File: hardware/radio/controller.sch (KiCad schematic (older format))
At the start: 11 parts, among them IC301 ATMEGA328-P, Q301 Q_NMOS_DGS, X301 8MHz

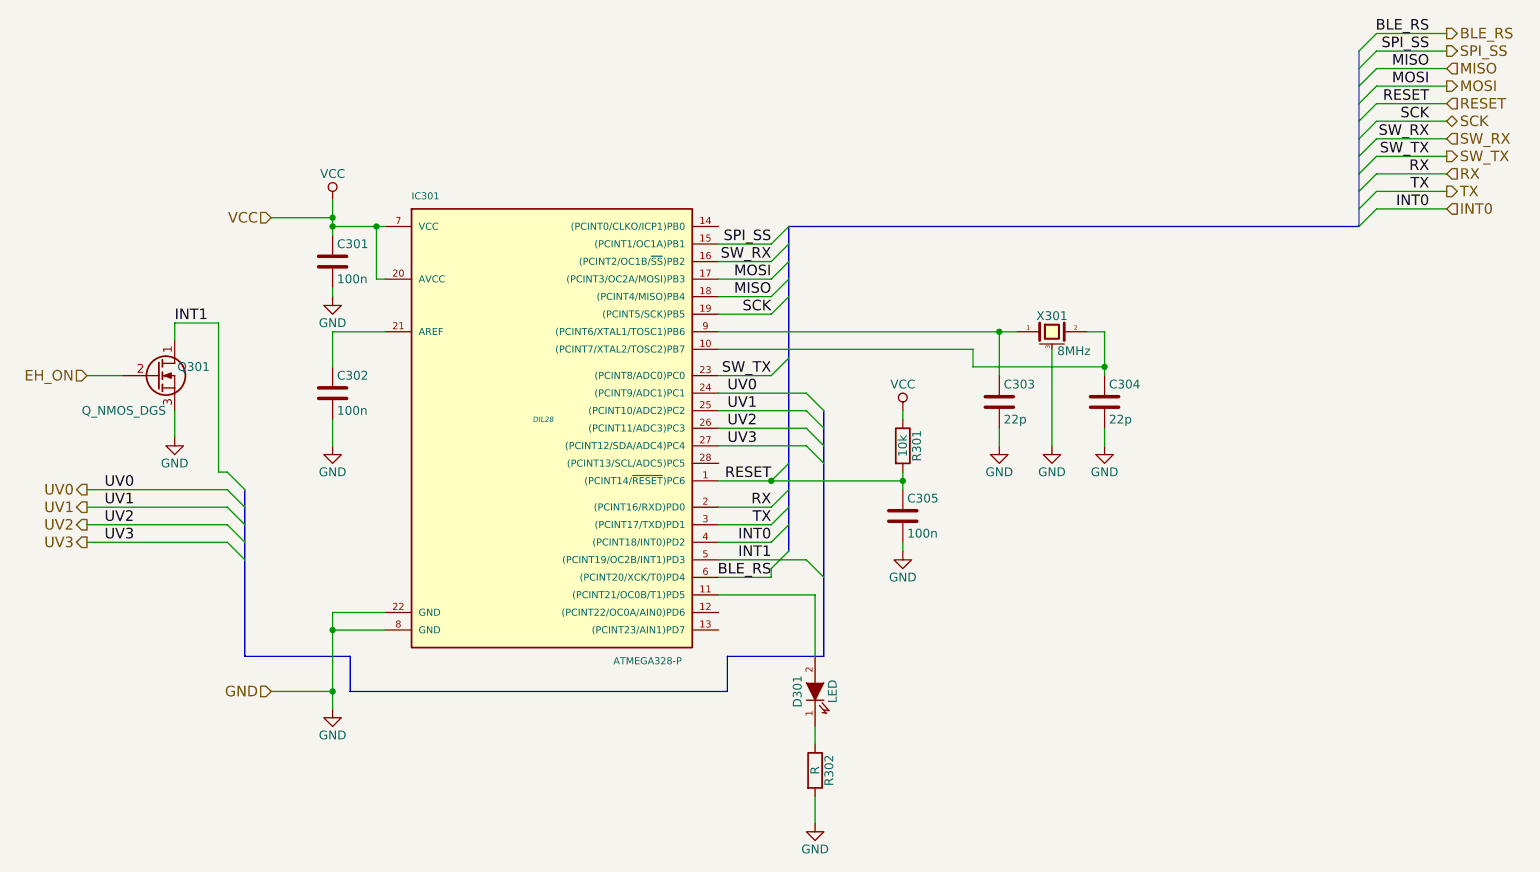
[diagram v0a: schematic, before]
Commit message: Work on PCB
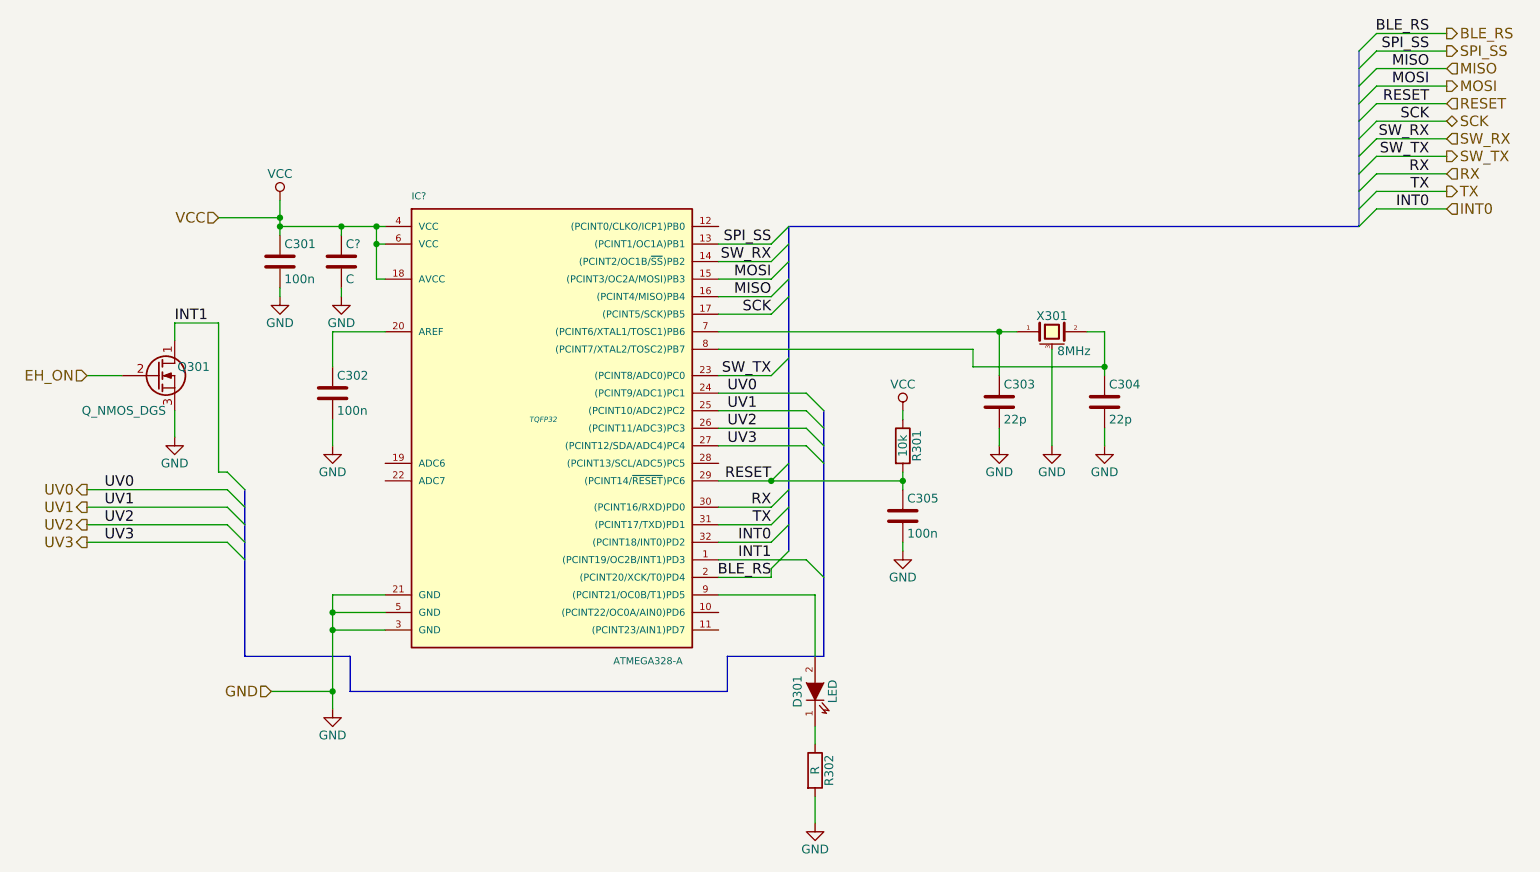
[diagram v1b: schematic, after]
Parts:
- removed IC301: ATMEGA328-P, DIL28, symbol ATMEGA328-P
- added C?: C, symbol C
- added IC?: ATMEGA328-A, TQFP32, symbol ATMEGA328-A
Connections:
- net BLE_RS: now also IC?.2 ((PCINT20/XCK/T0)PD4)
- net GND: now also C?.2, IC?.21 (GND), IC?.3 (GND), IC?.5 (GND)
- net INT0: now also IC?.32 ((PCINT18/INT0)PD2)
- net INT1: now also IC?.1 ((PCINT19/OC2B/INT1)PD3)
- net MISO: now also IC?.16 ((PCINT4/MISO)PB4)
- net MOSI: now also IC?.15 ((PCINT3/OC2A/MOSI)PB3)
- net RESET: now also IC?.29 ((PCINT14/~RESET~)PC6)
- net RX: now also IC?.30 ((PCINT16/RXD)PD0)
- net SCK: now also IC?.17 ((PCINT5/SCK)PB5)
- net SPI_SS: now also IC?.13 ((PCINT1/OC1A)PB1)
- net SW_RX: now also IC?.14 ((PCINT2/OC1B/~SS~)PB2)
- net SW_TX: now also IC?.23 ((PCINT8/ADC0)PC0)
- net TX: now also IC?.31 ((PCINT17/TXD)PD1)
- net UV0: now also IC?.24 ((PCINT9/ADC1)PC1)
- net UV1: now also IC?.25 ((PCINT10/ADC2)PC2)
- net UV2: now also IC?.26 ((PCINT11/ADC3)PC3)
- net UV3: now also IC?.27 ((PCINT12/SDA/ADC4)PC4)
- net VCC: now also C?.1, IC?.18 (AVCC), IC?.4 (VCC), IC?.6 (VCC)
- net at C304.1, X301.2: now also IC?.8 ((PCINT7/XTAL2/TOSC2)PB7)
- net at D301.2 (A): now also IC?.9 ((PCINT21/OC0B/T1)PD5)
- net at C302.1: now also IC?.20 (AREF)
- net at C303.1, X301.1: now also IC?.7 ((PCINT6/XTAL1/TOSC1)PB6)
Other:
- moved on the sheet: C301
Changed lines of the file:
@@
 $EndDescr
-$Comp
-L ATMEGA328-P IC301
-U 1 1 55EA8691
-P 4400 3100
-F 0 "IC301" H 3650 4350 40  0000 L BNN
-F 1 "ATMEGA328-P" H 4800 1700 40  0000 L BNN
-F 2 "DIL28" H 4400 3100 30  0000 C CIN
-F 3 "" H 4400 3100 60  0000 C CNN
-	1    4400 3100
-	1    0    0    -1
-$EndComp
 $Comp
 L CRYSTAL_SMD X301
@@
 $EndComp
 $Comp
-L GND #PWR308
+L GND #PWR028
 U 1 1 55EA8C66
 P 7600 3250
-F 0 "#PWR308" H 7600 3000 50  0001 C CNN
+F 0 "#PWR028" H 7600 3000 50  0001 C CNN
 F 1 "GND" H 7600 3100 50  0000 C CNN
 F 2 "" H 7600 3250 60  0000 C CNN
@@
 $EndComp
 $Comp
-L GND #PWR307
+L GND #PWR029
 U 1 1 55EA8C82
 P 7300 3250
-F 0 "#PWR307" H 7300 3000 50  0001 C CNN
+F 0 "#PWR029" H 7300 3000 50  0001 C CNN
 F 1 "GND" H 7300 3100 50  0000 C CNN
 F 2 "" H 7300 3250 60  0000 C CNN
@@
 $EndComp
 $Comp
-L GND #PWR306
+L GND #PWR030
 U 1 1 55EA8C9E
 P 7000 3250
-F 0 "#PWR306" H 7000 3000 50  0001 C CNN
+F 0 "#PWR030" H 7000 3000 50  0001 C CNN
 F 1 "GND" H 7000 3100 50  0000 C CNN
 F 2 "" H 7000 3250 60  0000 C CNN
@@
 $EndComp
 $Comp
-L VCC #PWR303
+L VCC #PWR031
 U 1 1 55EA9129
 P 6450 3050
-F 0 "#PWR303" H 6450 2900 50  0001 C CNN
+F 0 "#PWR031" H 6450 2900 50  0001 C CNN
 F 1 "VCC" H 6450 3200 50  0000 C CNN
 F 2 "" H 6450 3050 60  0000 C CNN
@@
 $EndComp
 $Comp
-L GND #PWR309
+L GND #PWR032
 U 1 1 55EA91E9
 P 6450 3850
-F 0 "#PWR309" H 6450 3600 50  0001 C CNN
+F 0 "#PWR032" H 6450 3600 50  0001 C CNN
 F 1 "GND" H 6450 3700 50  0000 C CNN
 F 2 "" H 6450 3850 60  0000 C CNN
@@
 TX
 $Comp
-L GND #PWR310
+L GND #PWR033
 U 1 1 55EA9D7E
 P 3200 4750
-F 0 "#PWR310" H 3200 4500 50  0001 C CNN
+F 0 "#PWR033" H 3200 4500 50  0001 C CNN
 F 1 "GND" H 3200 4600 50  0000 C CNN
 F 2 "" H 3200 4750 60  0000 C CNN
@@
 $EndComp
 $Comp
-L GND #PWR305
+L GND #PWR034
 U 1 1 55EA9F10
 P 3200 3250
-F 0 "#PWR305" H 3200 3000 50  0001 C CNN
+F 0 "#PWR034" H 3200 3000 50  0001 C CNN
 F 1 "GND" H 3200 3100 50  0000 C CNN
 F 2 "" H 3200 3250 60  0000 C CNN
@@
 $EndComp
 $Comp
-L VCC #PWR301
+L VCC #PWR035
 U 1 1 55EAA1EE
-P 3200 1850
-F 0 "#PWR301" H 3200 1700 50  0001 C CNN
-F 1 "VCC" H 3200 2000 50  0000 C CNN
-F 2 "" H 3200 1850 60  0000 C CNN
-F 3 "" H 3200 1850 60  0000 C CNN
-	1    3200 1850
+P 2900 1850
+F 0 "#PWR035" H 2900 1700 50  0001 C CNN
+F 1 "VCC" H 2900 2000 50  0000 C CNN
+F 2 "" H 2900 1850 60  0000 C CNN
+F 3 "" H 2900 1850 60  0000 C CNN
+	1    2900 1850
 	1    0    0    -1
 $EndComp
@@
 L C C301
 U 1 1 55EAA2CA
-P 3200 2200
-F 0 "C301" H 3225 2300 50  0000 L CNN
-F 1 "100n" H 3225 2100 50  0000 L CNN
-F 2 "" H 3238 2050 30  0000 C CNN
-F 3 "" H 3200 2200 60  0000 C CNN
-	1    3200 2200
-	1    0    0    -1
-$EndComp
-$Comp
-L GND #PWR302
+P 2900 2200
+F 0 "C301" H 2925 2300 50  0000 L CNN
+F 1 "100n" H 2925 2100 50  0000 L CNN
+F 2 "" H 2938 2050 30  0000 C CNN
+F 3 "" H 2900 2200 60  0000 C CNN
+	1    2900 2200
+	1    0    0    -1
+$EndComp
+$Comp
+L GND #PWR036
 U 1 1 55EAA376
-P 3200 2400
-F 0 "#PWR302" H 3200 2150 50  0001 C CNN
-F 1 "GND" H 3200 2250 50  0000 C CNN
-F 2 "" H 3200 2400 60  0000 C CNN
-F 3 "" H 3200 2400 60  0000 C CNN
-	1    3200 2400
+P 2900 2400
+F 0 "#PWR036" H 2900 2150 50  0001 C CNN
+F 1 "GND" H 2900 2250 50  0000 C CNN
+F 2 "" H 2900 2400 60  0000 C CNN
+F 3 "" H 2900 2400 60  0000 C CNN
+	1    2900 2400
 	1    0    0    -1
 $EndComp
@@
 Text HLabel 2850 4650 0    60   Input ~ 0
 GND
-Text HLabel 2850 1950 0    60   Input ~ 0
+Text HLabel 2550 1950 0    60   Input ~ 0
 VCC
 $Comp
@@
 $EndComp
 $Comp
-L GND #PWR311
+L GND #PWR037
 U 1 1 55EACDAA
 P 5950 5400
-F 0 "#PWR311" H 5950 5150 50  0001 C CNN
+F 0 "#PWR037" H 5950 5150 50  0001 C CNN
 F 1 "GND" H 5950 5250 50  0000 C CNN
 F 2 "" H 5950 5400 60  0000 C CNN
@@
 $EndComp
 $Comp
-L GND #PWR304
+L GND #PWR038
 U 1 1 55EAF28A
 P 2300 3200
-F 0 "#PWR304" H 2300 2950 50  0001 C CNN
+F 0 "#PWR038" H 2300 2950 50  0001 C CNN
 F 1 "GND" H 2300 3050 50  0000 C CNN
 F 2 "" H 2300 3200 60  0000 C CNN
@@
 	3500 4200 3200 4200
 Wire Wire Line
-	3200 4200 3200 4750
+	3200 4100 3200 4750
 Wire Wire Line
 	3500 4300 3200 4300
 Connection ~ 3200 4300
 Wire Wire Line
-	3500 2300 3450 2300
-Wire Wire Line
-	3450 2300 3450 2000
-Wire Wire Line
-	3200 2000 3500 2000
+	3450 2300 3500 2300
+Wire Wire Line
+	3450 2000 3450 2300
+Wire Wire Line
+	2900 2000 3500 2000
 Connection ~ 3450 2000
 Wire Wire Line
@@
 	3200 3100 3200 3250
 Wire Wire Line
-	3200 1850 3200 2050
-Connection ~ 3200 2000
-Wire Wire Line
-	3200 2350 3200 2400
+	2900 1850 2900 2050
+Connection ~ 2900 2000
+Wire Wire Line
+	2900 2350 2900 2400
 Wire Bus Line
 	9050 1000 9050 2000
@@
 	9150 1900 9550 1900
 Wire Wire Line
-	3200 1950 2850 1950
-Connection ~ 3200 1950
+	2900 1950 2550 1950
+Connection ~ 2900 1950
 Wire Wire Line
 	3200 4650 2850 4650
@@
 Text Label 5450 3250 0    60   ~ 0
 UV3
+$Comp
+L ATMEGA328-A IC?
+U 1 1 55ED2326
+P 4400 3100
+F 0 "IC?" H 3650 4350 40  0000 L BNN
+F 1 "ATMEGA328-A" H 4800 1700 40  0000 L BNN
+F 2 "TQFP32" H 4400 3100 30  0000 C CIN
+F 3 "" H 4400 3100 60  0000 C CNN
+	1    4400 3100
+	1    0    0    -1
+$EndComp
+Wire Wire Line
+	3500 2100 3450 2100
+Connection ~ 3450 2100
+Wire Wire Line
+	3500 4100 3200 4100
+Connection ~ 3200 4200
+$Comp
+L C C?
+U 1 1 55ED2949
+P 3250 2200
+F 0 "C?" H 3275 2300 50  0000 L CNN
+F 1 "C" H 3275 2100 50  0000 L CNN
+F 2 "" H 3288 2050 30  0000 C CNN
+F 3 "" H 3250 2200 60  0000 C CNN
+	1    3250 2200
+	1    0    0    -1
+$EndComp
+Wire Wire Line
+	3250 2000 3250 2050
+Connection ~ 3250 2000
+Wire Wire Line
+	3250 2350 3250 2400
+$Comp
+L GND #PWR?
+U 1 1 55ED2A96
+P 3250 2400
+F 0 "#PWR?" H 3250 2150 50  0001 C CNN
+F 1 "GND" H 3250 2250 50  0000 C CNN
+F 2 "" H 3250 2400 60  0000 C CNN
+F 3 "" H 3250 2400 60  0000 C CNN
+	1    3250 2400
+	1    0    0    -1
+$EndComp
 $EndSCHEMATC
